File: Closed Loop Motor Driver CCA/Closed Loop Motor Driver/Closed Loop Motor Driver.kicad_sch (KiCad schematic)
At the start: 14 parts, among them J1 JST 1x4, J2 JST 1X6, J3 HEADER 1x7 socket, J4 Conn_01x03_Pin, J5 Screw_Terminal_01x03, J6 Screw_Terminal_01x02, J7 JST 1x4, J8 Conn_02x05_Counter_Clockwise, SW1 SW_Push, U1 RPI PICO, U7 TXB0108DQSR

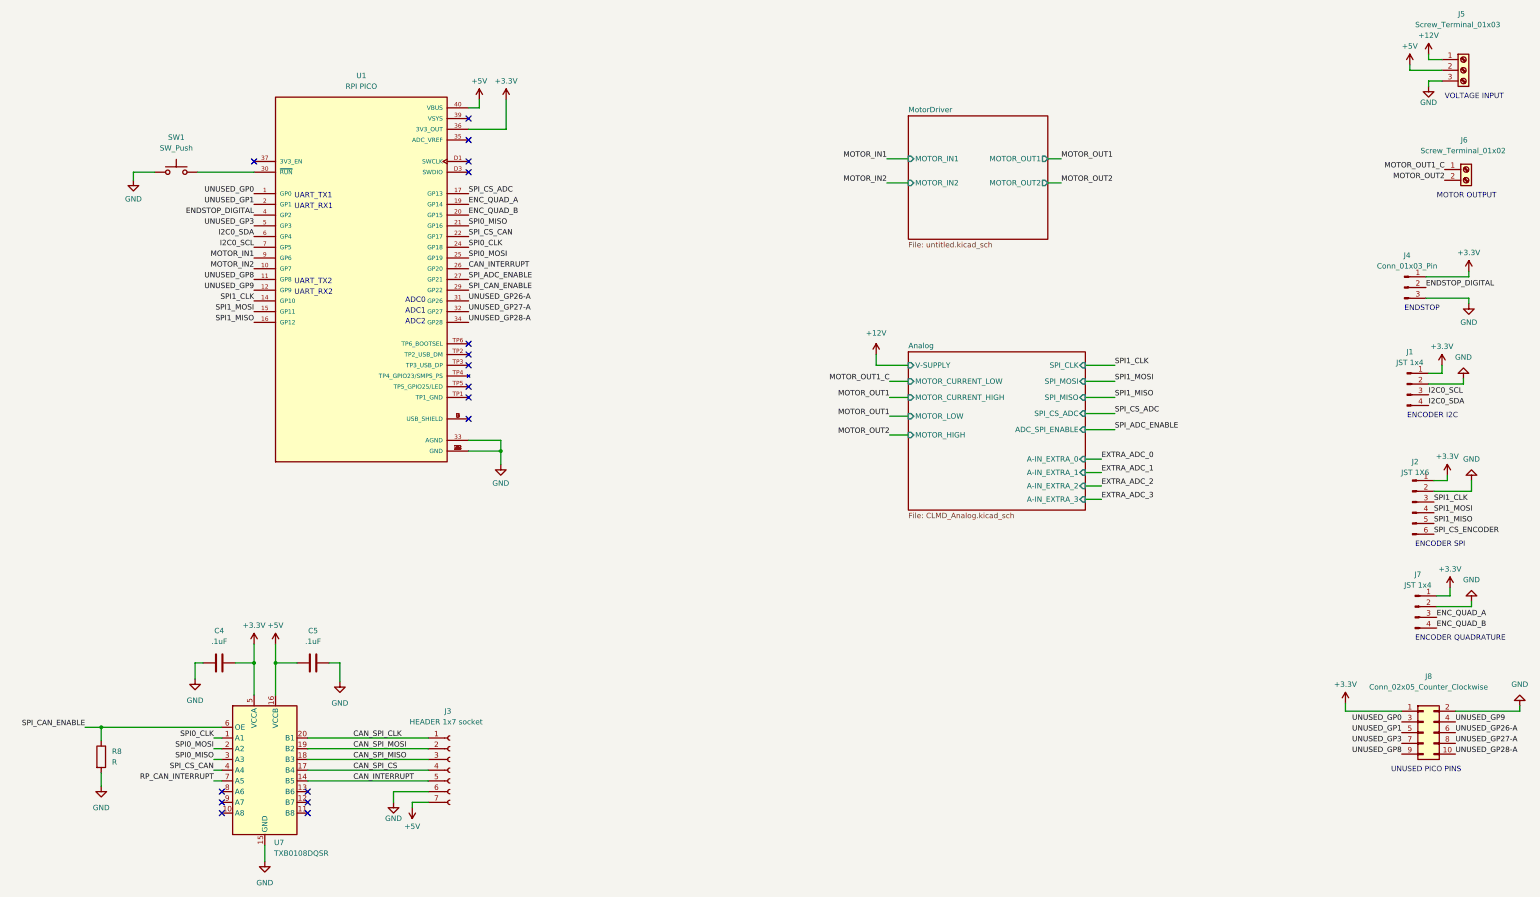
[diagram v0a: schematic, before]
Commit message: driver updates
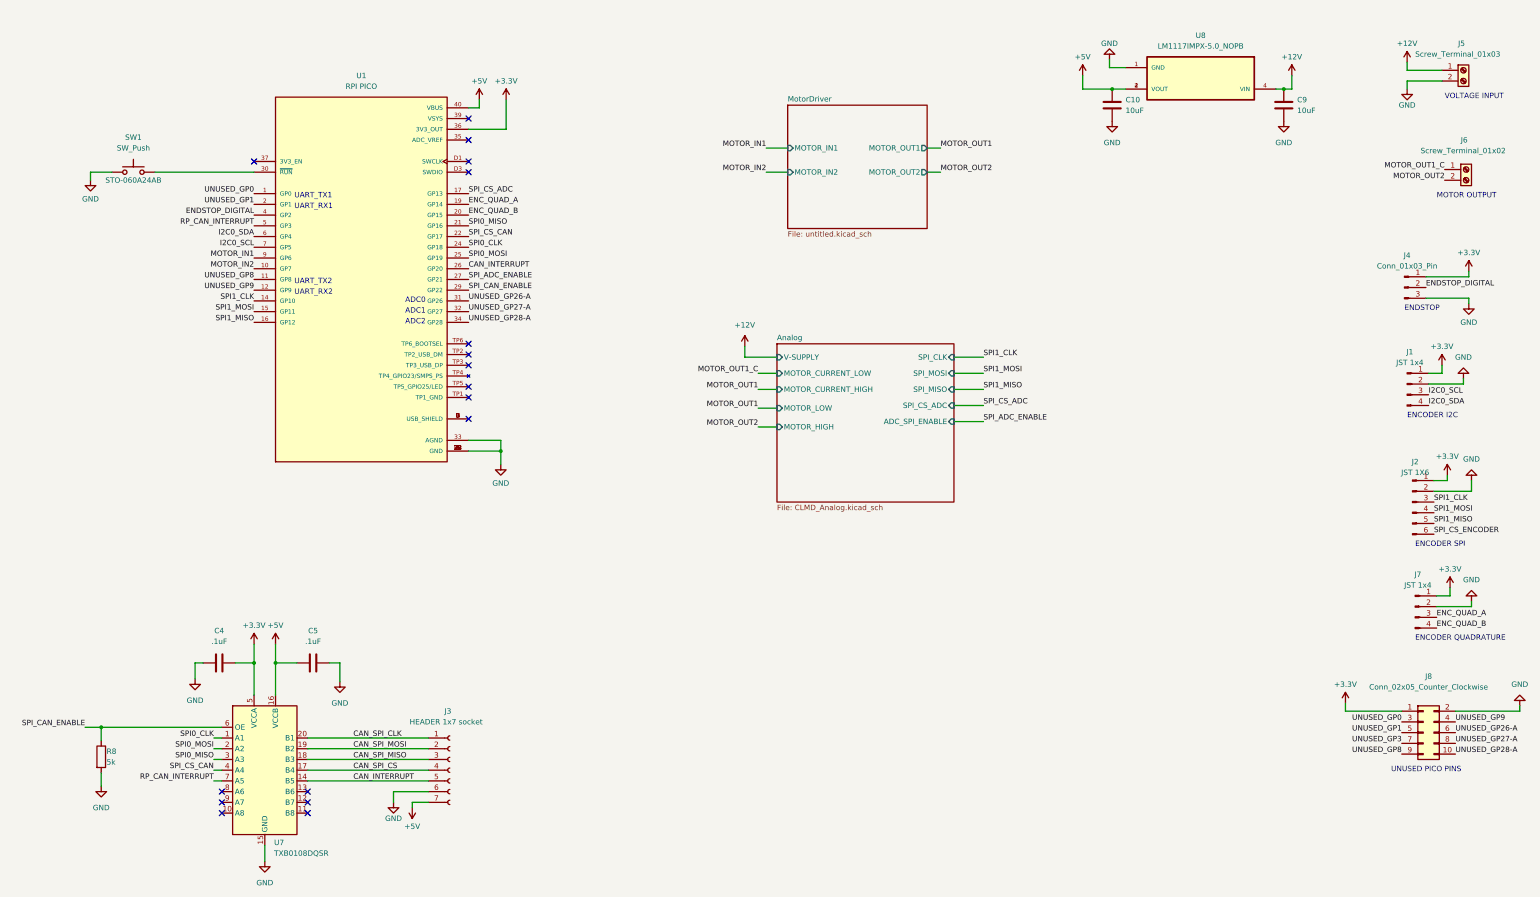
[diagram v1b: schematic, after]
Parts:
- added C10, C9: 10uF, symbol Device:C
- added U8: LM1117IMPX-5.0_NOPB, LM1117IMPX-5.0_NOPB:SOT230P700X180-4N, symbol LM1117IMPX-5.0_NOPB:LM1117IMPX-5.0_NOPB
- J5: symbol Connector:Screw_Terminal_01x03 -> Connector:Screw_Terminal_01x02
- R8: value R -> 5k; PART_NO (none) -> 1879246-3
- SW1: PART_NO (none) -> STO-060A24AB
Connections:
- net +12V: now also C9.1, U8.4 (VOUT)
- net +5V: now also C10.1, U8.2 (VOUT), U8.4 (VOUT); no longer J5.2 (Pin_2)
- net GND: now also J5.2 (Pin_2), C10.2, C9.2, U8.1 (GND); no longer J5.3 (Pin_3)
- net RP_CAN_INTERRUPT: now also U1.5 (GP3)
- net UNUSED_GP3: no longer U1.5 (GP3)
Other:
- sheet Analog ports: added none; removed A-IN_EXTRA_0, A-IN_EXTRA_1, A-IN_EXTRA_2, A-IN_EXTRA_3
- moved on the sheet: SW1
